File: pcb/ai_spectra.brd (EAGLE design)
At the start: 127 x 127 mm, 97 parts, among them IC1 ATMEGA328P-PDIP, J1 1X06, J3 1X02ST, U1 MC7805-HOR, U2 TLC2262

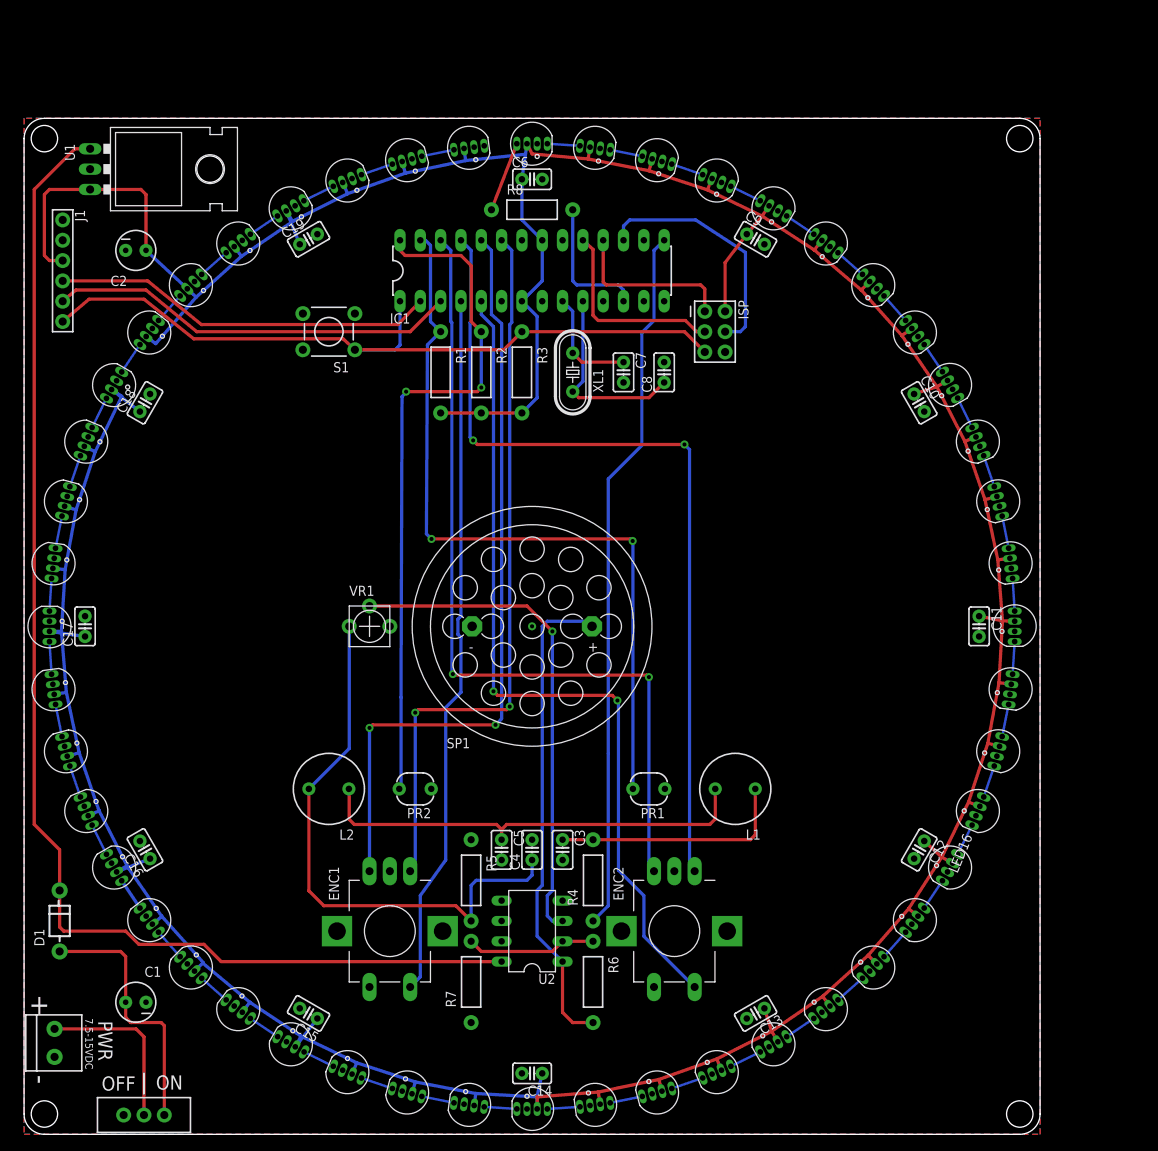
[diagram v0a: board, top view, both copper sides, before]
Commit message: adding gerbers
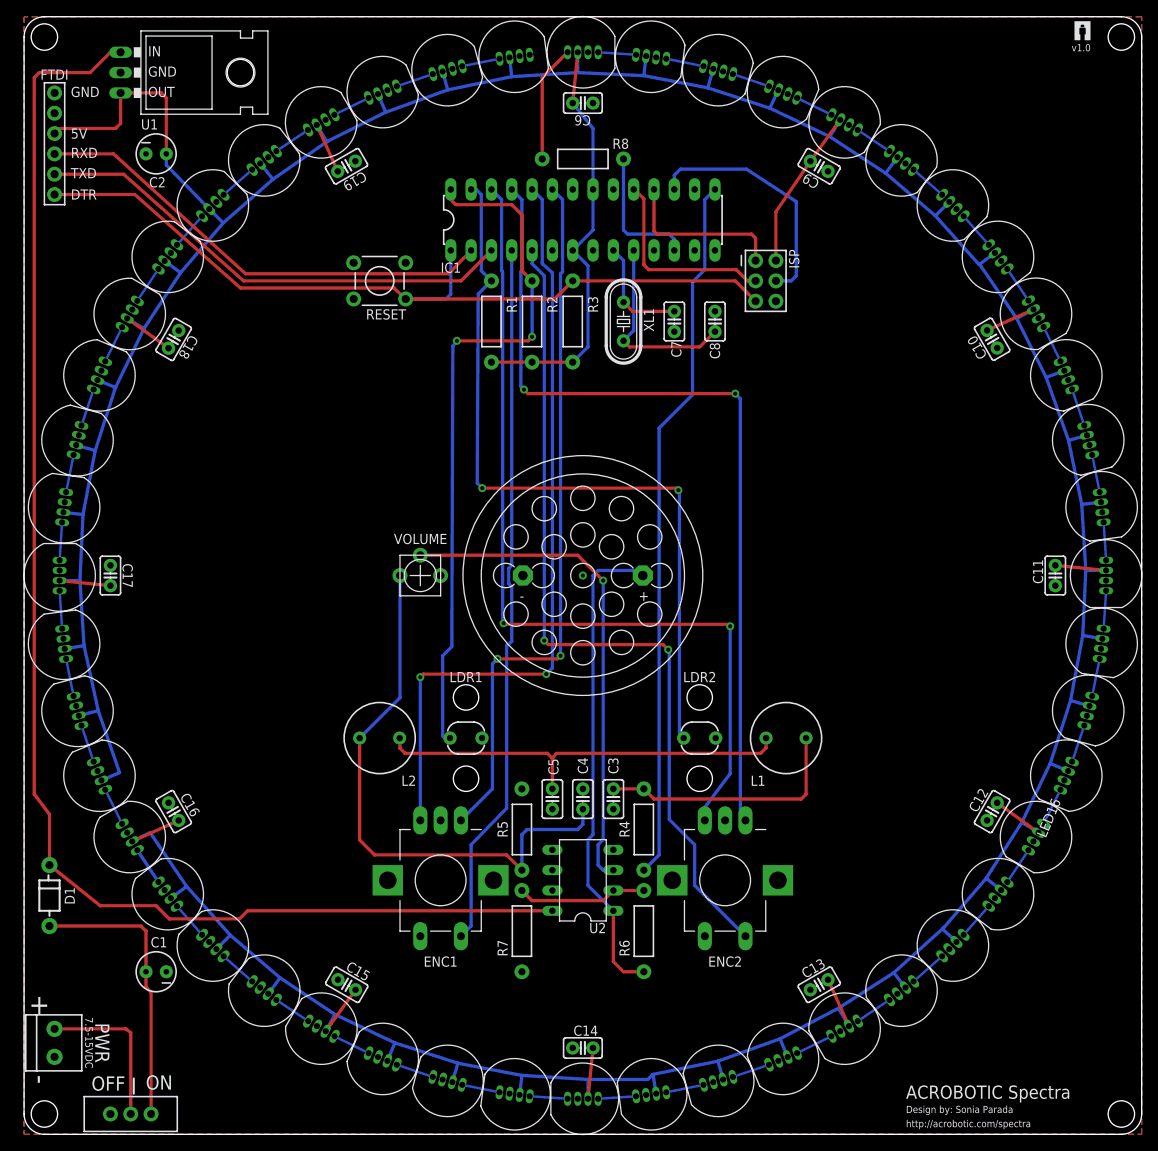
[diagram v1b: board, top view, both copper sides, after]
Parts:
- removed J1: 1X06, Ai_Connectors:1X06
- removed PR1, PR2: LDR-PTH, Ai_Sensors:LDR
- removed S1: SW-SPSTTH06X06, Ai_Electromechanical:SW-SPST-TH06X06
- removed VR1: 10K, Ai_Passives:POT-05X05
- added FTDI: 1X06, Ai_Connectors:1X06
- added LDR1, LDR2: LDR-PTH, Ai_Sensors:LDR
- added RESET: SW-SPSTTH06X06, Ai_Electromechanical:SW-SPST-TH06X06
- added U$18: AI-LOGOXS, Ai_Miscellany:AI-LOGO-XS
- added VOLUME: 10K, Ai_Passives:POT-05X05
- LED1, LED10, LED11, LED12, LED13, LED14, LED15, LED16, LED17, LED18, LED19, LED2, LED20, LED21, LED22, LED23, LED24, LED25, LED26, LED27, LED28, LED29, LED3, LED30, LED31, LED32, LED33, LED34, LED35, LED36, LED37, LED38, LED39, LED4, LED40, LED41, LED42, LED43, LED44, LED45, LED46, LED47, LED48, LED5, LED6, LED7, LED8, LED9: value LED-PL9823-F5 -> LED-PL9823-F8; device Ai_LED:LED-PL9823-F5 -> Ai_LED:LED-PL9823-F8
- moved STANDOFF3 18.0 mm to (137.2, 137.2)
- moved LED7 14.1 mm to (116.1, 116.1)
- moved LED6 14.0 mm to (109.7, 121.7)
- moved LED8 14.0 mm to (121.7, 109.7)
- moved LED5 13.9 mm to (102.6, 126.5)
- moved LED9 13.9 mm to (126.5, 102.6)
- moved LED10 13.8 mm to (130.3, 94.9)
- moved LED4 13.8 mm to (94.9, 130.3)
- moved LED11 13.6 mm to (133.0, 86.8)
- moved LED3 13.6 mm to (86.8, 133.0)
- moved LED12 13.4 mm to (134.7, 78.4)
- moved LED2 13.4 mm to (78.4, 134.7)
- moved LED1 13.1 mm to (69.8, 135.3)
- moved LED13 13.1 mm to (135.3, 69.8)
- moved LED14 12.7 mm to (134.7, 61.3)
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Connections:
- net 5V: now also FTDI.3; no longer J1.3
- net GND: now also FTDI.1, LDR1.1, LDR2.1, RESET.A@1, VOLUME.3; no longer J1.1, PR1.1, PR2.1, S1.A@1, VR1.3
- net LDR1: now also LDR2.2; no longer PR1.2
- net LDR2: now also LDR1.2; no longer PR2.2
- net N$1: now also VOLUME.2; no longer VR1.2
- net RESET: now also FTDI.6, RESET.B@1; no longer J1.6, S1.B@1
- net RXI: now also FTDI.4; no longer J1.4
- net SND_CLN: now also VOLUME.1; no longer VR1.1
- net TXO: now also FTDI.5; no longer J1.5
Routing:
- net 5V: track 571.5 -> 676.1 mm
- net VDD: track 159.6 -> 176.9 mm
- net RXI: track 47.9 -> 59.1 mm
- net TXO: track 51.2 -> 61.3 mm
- net RESET: track 96.9 -> 106.0 mm
- net D: track 8.84 -> 14.7 mm
- net ENC2_B: track 104.0 -> 109.4 mm
- net VIN: track 32.6 -> 35.5 mm
- net N$13: track 55.7 -> 53.2 mm
- net ENC1_A: track 91.1 -> 89.0 mm
- net N$12: track 30.1 -> 31.9 mm
- net N$5: track 21.4 -> 19.9 mm
- net LDR2: track 86.2 -> 87.4 mm
- net N$42: track 4.07 -> 4.75 mm
- net N$38: track 4.07 -> 4.75 mm
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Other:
- board size 127 x 127 mm -> 139.7 x 139.7 mm
- board text added: "5V"
- board text added: "ACROBOTIC Spectra"
- board text added: "DTR"
- board text added: "Design by: Sonia Parada"
- board text added: "GND"
- board text added: "IN"
- board text added: "OUT"
- board text added: "RXD"
- board text added: "TXD"
- board text added: "http://acrobotic.com/spectra"
- board text added: "v1.0"
